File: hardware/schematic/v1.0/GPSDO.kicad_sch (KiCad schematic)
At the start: 61 parts, among them J1 USB_C_Receptacle_USB2.0_16P, Q1 NMOS, SW1 SW_Push, U1 STM32G431KBUx, U2 OCXO-10M, U3 SKG123N, U4 IPEX1, U5 BQ25890, U6 TPS7A8901, U7 CH340E, Y1 Crystal_GND24

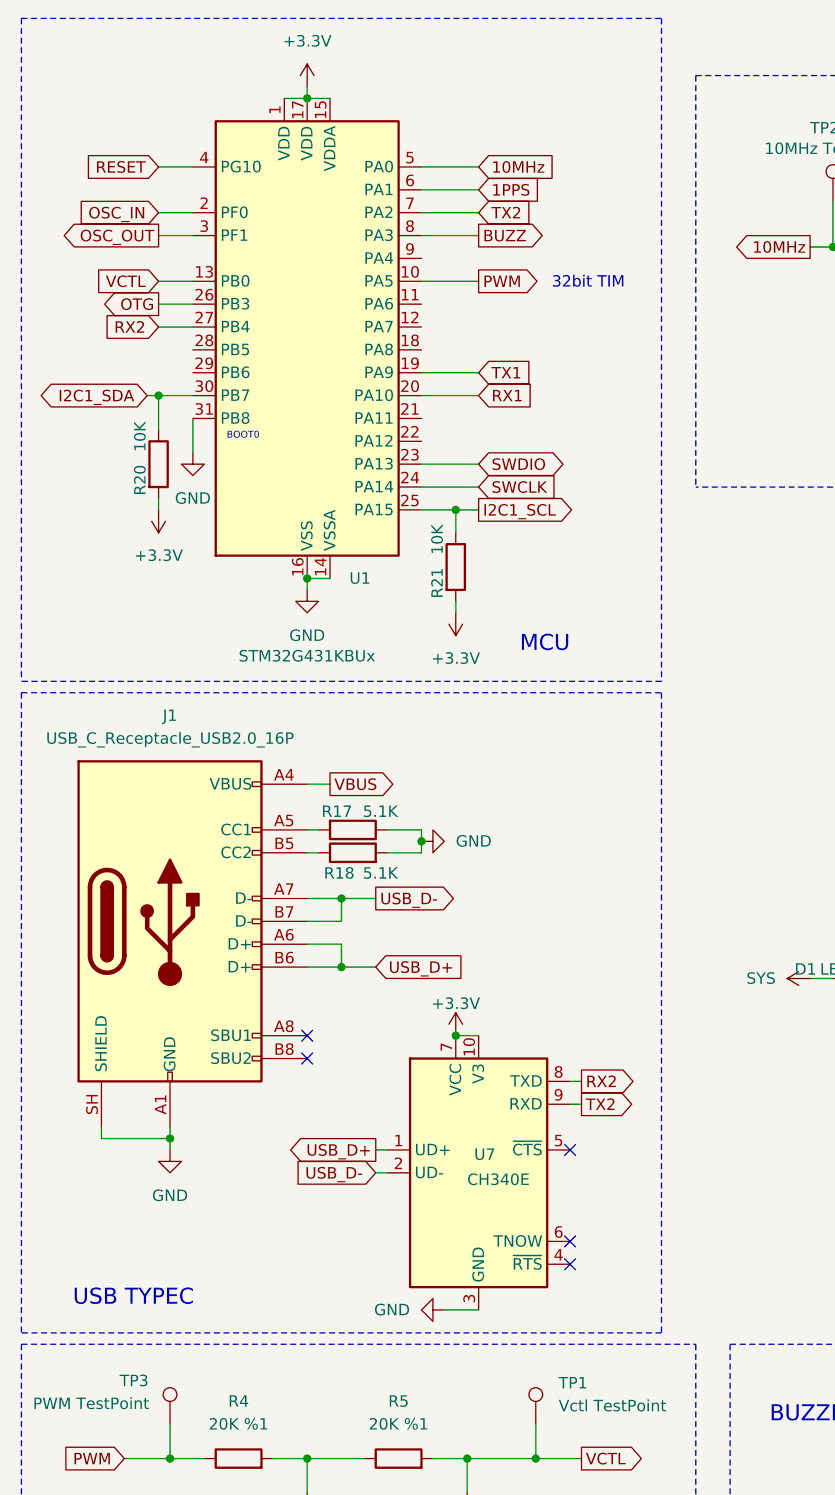
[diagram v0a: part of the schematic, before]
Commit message: 更新 GPSDO 硬件设计文件
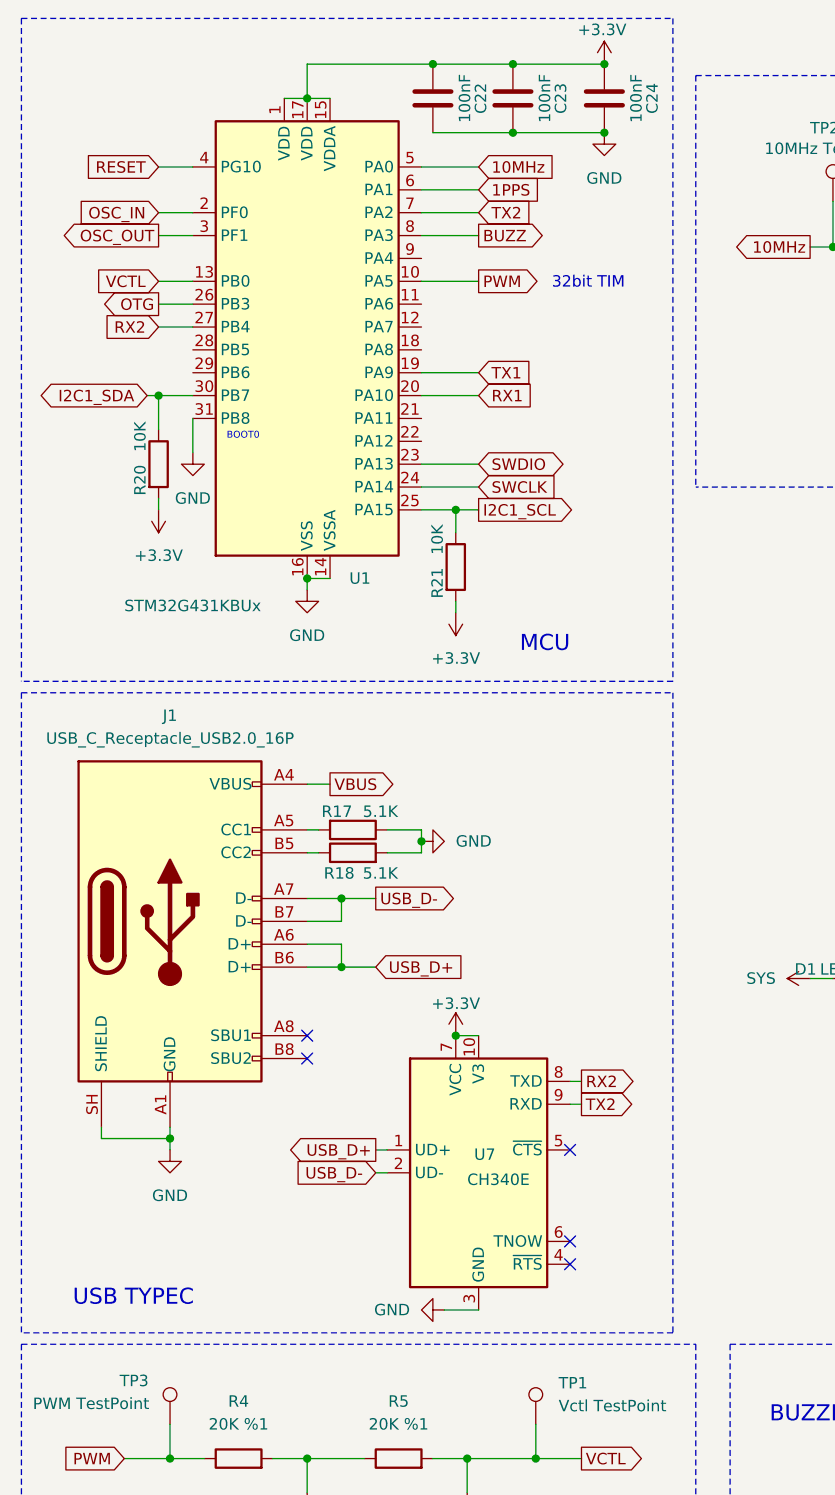
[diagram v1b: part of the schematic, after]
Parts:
- added C22, C23, C24: 100nF, Capacitor_SMD:C_0402_1005Metric, symbol Device:C
- C19, C20: footprint Capacitor_SMD:C_0603_1608Metric -> Capacitor_SMD:C_0402_1005Metric
- R14, R16, R17, R18, R20, R21: footprint Resistor_SMD:R_0603_1608Metric -> Resistor_SMD:R_0402_1005Metric
- SW1: footprint Capacitor_SMD:C_0201_0603Metric -> Button_Switch_SMD:SW_Tactile_SPST_NO_Straight_CK_PTS636Sx25SMTRLFS
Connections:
- net +3.3V: now also C22.1, C23.1, C24.1
- net BAT-: now also C22.2, C23.2, C24.2
